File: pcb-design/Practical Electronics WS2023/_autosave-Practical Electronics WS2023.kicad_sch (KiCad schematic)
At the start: 38 parts, among them IC1 SN74LVC2G04DBVT, J1 PWR Jack, J2 MIDI Input, J3 MIDI Thru out, J4 Conn_01x03, J5 ISP, Q1 Q_NMOS_DGS, SW1 SW_SPDT, SW2 SW_SPDT, SW4 SW_SPDT, U1 6N138, U2 ADP2303ARDZ-5.0, U3 ATmega328P-A, Y1 16Mhz Crystal

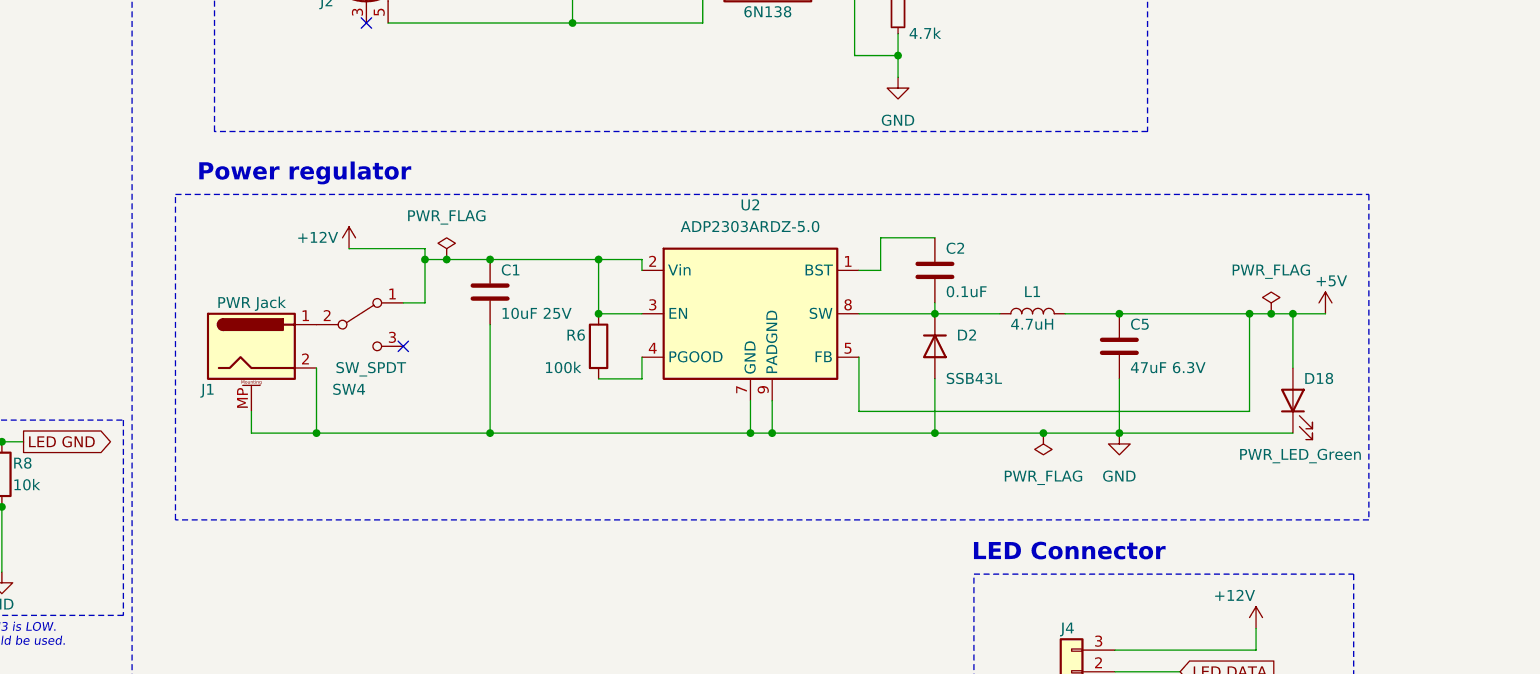
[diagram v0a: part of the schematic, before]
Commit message: Update schematic
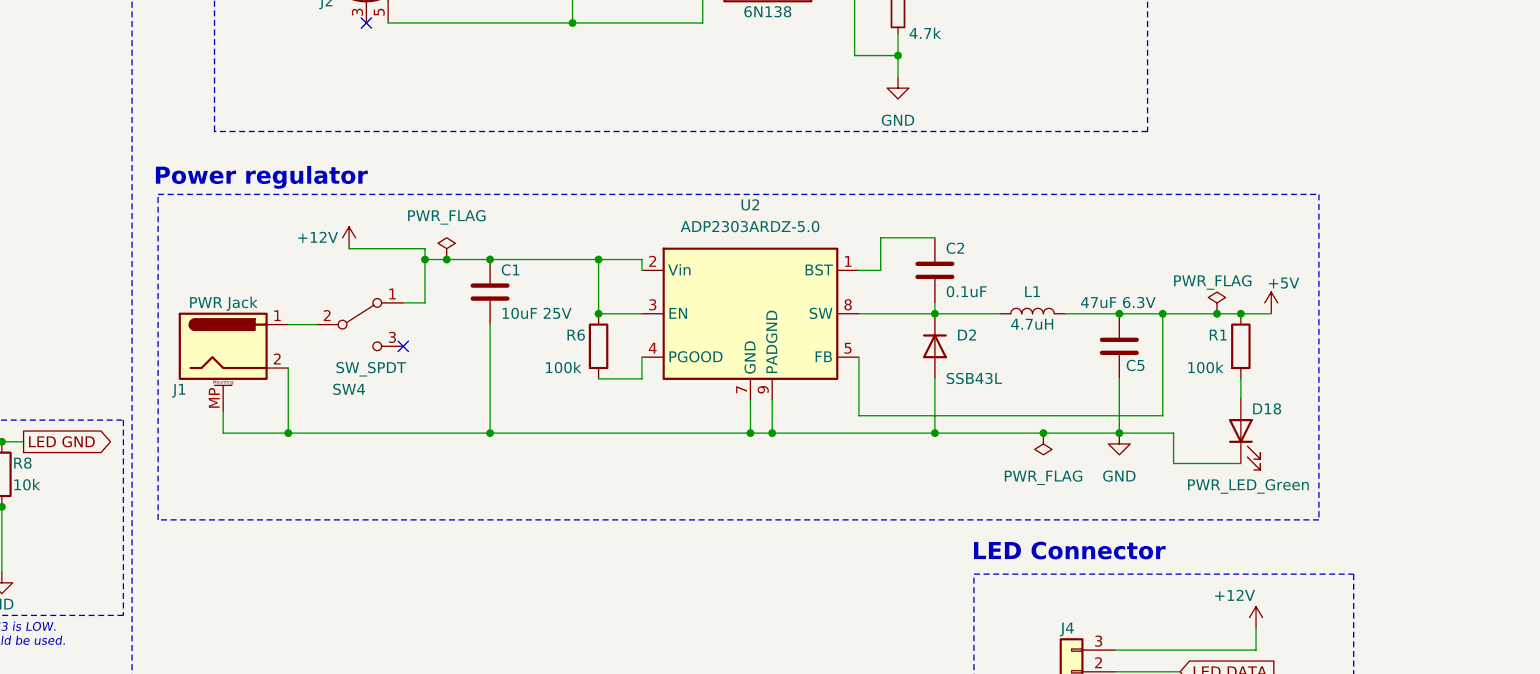
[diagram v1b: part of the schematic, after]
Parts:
- added R1: 100k, symbol Device:R
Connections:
- net +5V: now also R1.1; no longer D18.2 (A)
- new net: D18.2 (A), R1.2
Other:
- moved on the sheet: D18, J1
